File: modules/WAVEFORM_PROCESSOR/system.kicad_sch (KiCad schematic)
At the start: 8 parts, among them J1 Card_Connector, J2 Mono_Jack, J3 Mono_Jack, J4 Mono_Jack, J5 Mono_Jack

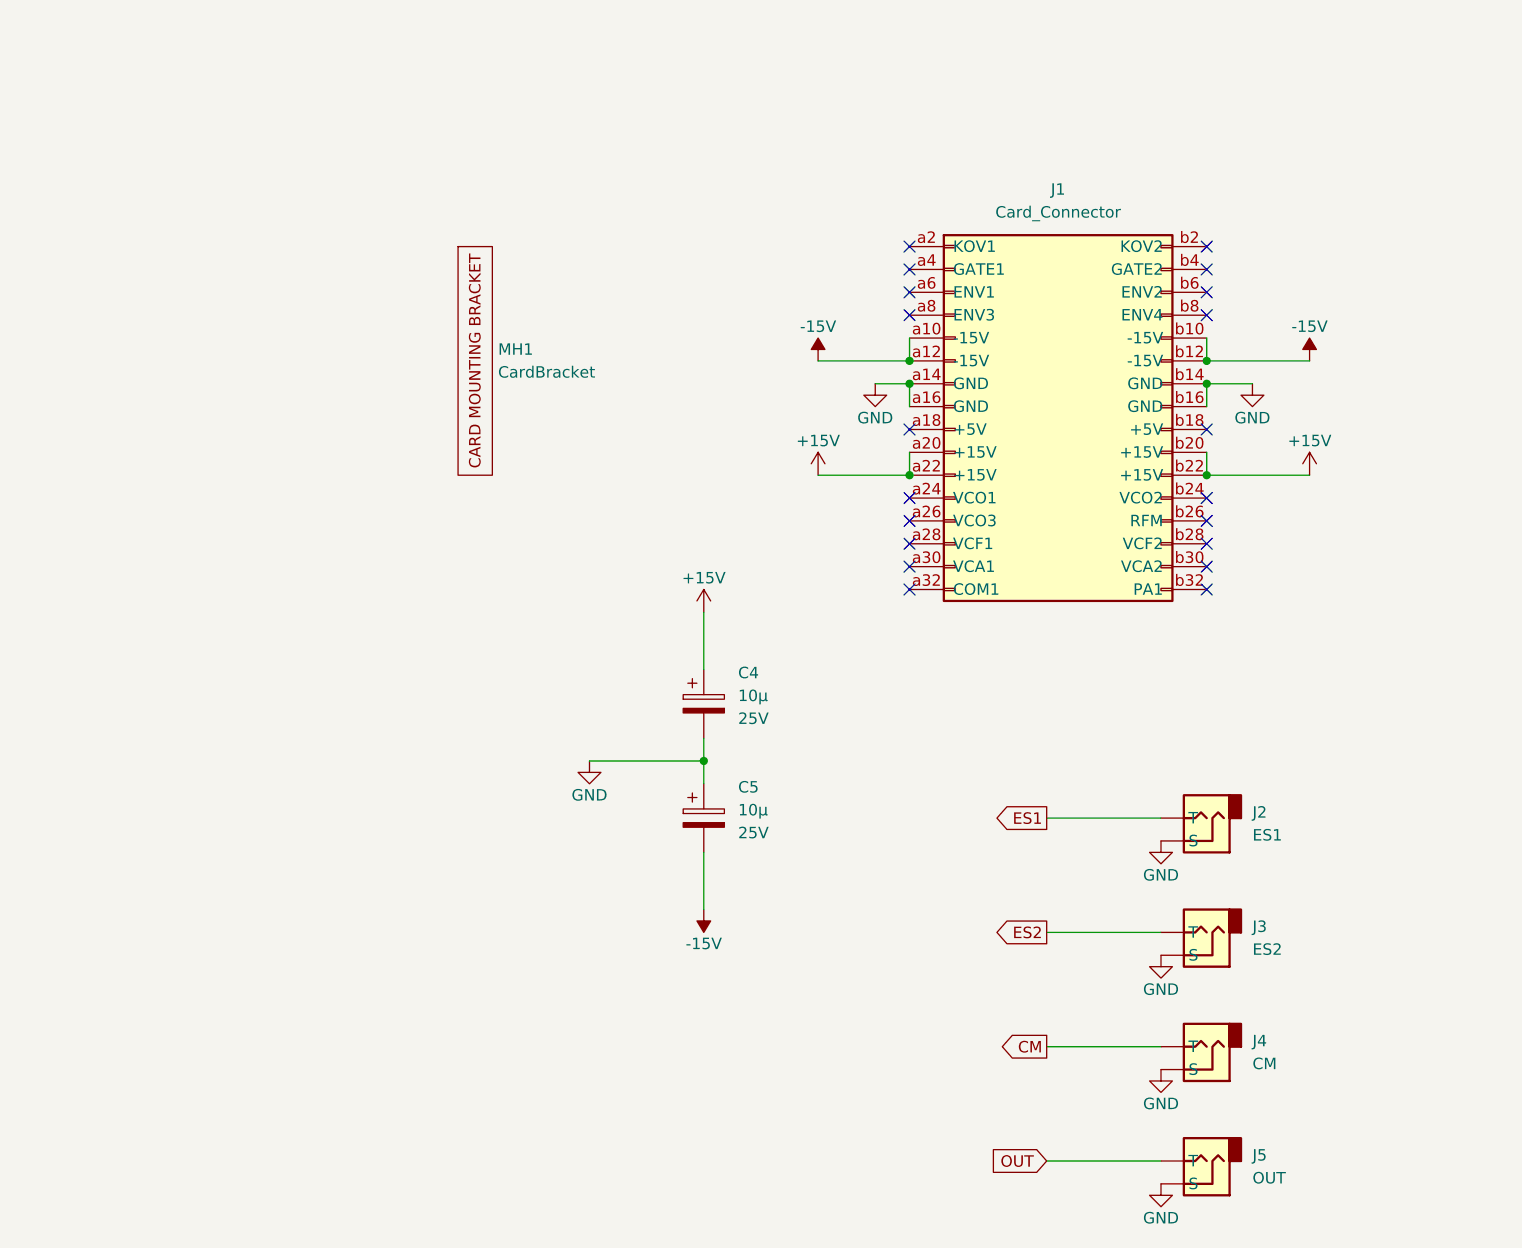
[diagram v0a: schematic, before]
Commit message: waveform processor updates
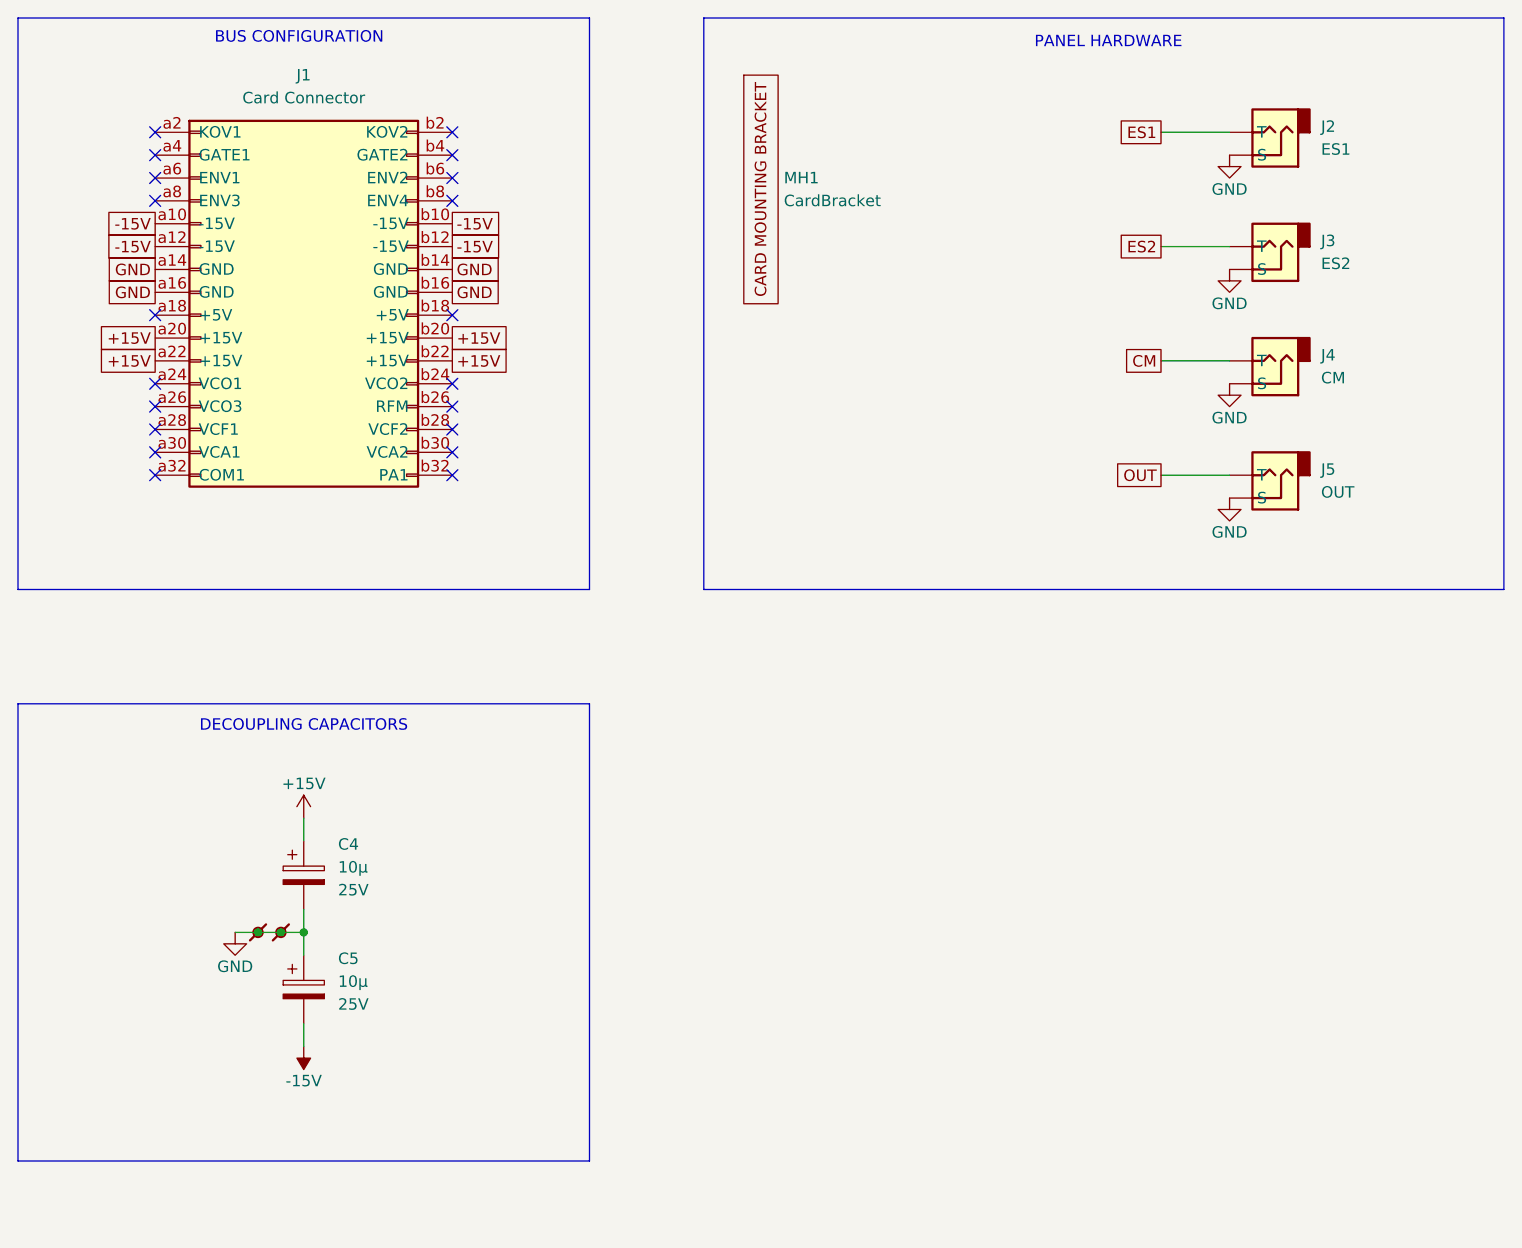
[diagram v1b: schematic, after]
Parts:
- added J7, J8: GND, FormantKO:Wire_1x01_D40mil_OD80mil, symbol FormantKO:WireConnector
- C4, C5: footprint FormantKO:CP_Axial_600 -> FormantKO:CP_Axial_P800mil
- J1: value Card_Connector -> Card Connector; footprint FormantKO:Card_Connector -> FormantKO:CardConnector; symbol FormantKO:Card_Connector -> FormantKO:CardConnector
- J2, J3, J4, J5: footprint FormantKO:Panel_Connector_1x02 -> FormantKO:PanelConnector_1x02; symbol FormantKO:Mono_Jack -> FormantKO:MonoJack
- MH1: footprint FormantKO:Card_Bracket -> FormantKO:CardBracket; symbol FormantKO:Card_Bracket -> FormantKO:CardBracket
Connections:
- net GND: now also J7.1, J8.1
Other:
- note added: "BUS CONFIGURATION"
- note added: "DECOUPLING CAPACITORS"
- note added: "PANEL HARDWARE"
- moved on the sheet: C4, C5, J1, J2, J3, J4, J5, MH1

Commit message: waveform process update
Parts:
- J7, J8: Spice_Model 0 -> (none); Spice_Primitive R -> (none)
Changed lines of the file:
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@@
 			)
 		)
-		(property "Spice_Primitive" "R"
+		(property "Sim.Device" "SPICE"
 			(at 55.245 125.73 0)
 			(hide yes)
@@
 			)
 		)
-		(property "Spice_Model" "0"
-			(at 52.705 128.905 0)
-			(hide yes)
-			(show_name no)
-			(do_not_autoplace no)
-			(effects
-				(font
-					(size 1.27 1.27)
-				)
-				(justify right top)
+		(property "Sim.Params" "type=\"R\" model=\"0\" lib=\"\""
+			(at 0 0 0)
+			(hide yes)
+			(show_name no)
+			(do_not_autoplace no)
+			(effects
+				(font
+					(size 1.27 1.27)
+				)
+			)
+		)
+		(property "Sim.Pins" "1=1"
+			(at 0 0 0)
+			(hide yes)
+			(show_name no)
+			(do_not_autoplace no)
+			(effects
+				(font
+					(size 1.27 1.27)
+				)
 			)
 		)
@@
 			)
 		)
-		(property "Spice_Primitive" "R"
+		(property "Sim.Device" "SPICE"
 			(at 52.705 125.73 0)
 			(hide yes)
@@
 			)
 		)
-		(property "Spice_Model" "0"
-			(at 50.165 128.905 0)
-			(hide yes)
-			(show_name no)
-			(do_not_autoplace no)
-			(effects
-				(font
-					(size 1.27 1.27)
-				)
-				(justify right top)
-			)
-		)
+		(property "Sim.Params" "type=\"R\" model=\"0\" lib=\"\""
+			(at 0 0 0)
+			(hide yes)
+			(show_name no)
+			(do_not_autoplace no)
+			(effects
+				(font
+					(size 1.27 1.27)
+				)
+			)
+		)
+		(property "Sim.Pins" "1=1"
+			(at 0 0 0)
+			(hide yes)
+			(show_name no)
+			(do_not_autoplace no)
+			(effects
+				(font
+					(size 1.27 1.27)
+				)
+			)
+		)

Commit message: mixer translation
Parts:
- C4, C5: footprint FormantKO:CP_Axial_P800mil -> FormantKO:CP_Axial_P600mil
- J7, J8: Spice_Model (none) -> 0; Spice_Primitive (none) -> R; now left out of the parts list
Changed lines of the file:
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@@
+			)
+		)
+		(property "Sim.Params" ""
+			(at 165.1 38.1 0)
+			(hide yes)
+			(show_name no)
+			(do_not_autoplace no)
+			(effects
+				(font
+					(size 1.27 1.27)
+				)
 			)
 		)
@@
 			)
 		)
+		(property "Sim.Params" ""
+			(at 165.1 76.2 0)
+			(hide yes)
+			(show_name no)
+			(do_not_autoplace no)
+			(effects
+				(font
+					(size 1.27 1.27)
+				)
+			)
+		)
 		(pin "1"
 		)
@@
 			)
 		)
+		(property "Sim.Params" ""
+			(at 165.1 63.5 0)
+			(hide yes)
+			(show_name no)
+			(do_not_autoplace no)
+			(effects
+				(font
+					(size 1.27 1.27)
+				)
+			)
+		)
 		(pin "1"
 		)
@@
 			)
 		)
+		(property "Sim.Params" ""
+			(at 107.95 44.45 0)
+			(hide yes)
+			(show_name no)
+			(do_not_autoplace no)
+			(effects
+				(font
+					(size 1.27 1.27)
+				)
+			)
+		)
 		(instances
 			(project "WAVEFORM_PROCESSOR"
@@
 			)
 		)
+		(property "Sim.Params" ""
+			(at 165.1 50.8 0)
+			(hide yes)
+			(show_name no)
+			(do_not_autoplace no)
+			(effects
+				(font
+					(size 1.27 1.27)
+				)
+			)
+		)
 		(pin "1"
 		)
@@
 		(body_style 1)
 		(exclude_from_sim no)
-		(in_bom yes)
+		(in_bom no)
 		(on_board yes)
 		(in_pos_files yes)
@@
 			)
 		)
-		(property "Sim.Device" "SPICE"
+		(property "Spice_Primitive" "R"
 			(at 55.245 125.73 0)
 			(hide yes)
@@
 			)
 		)
-		(property "Sim.Params" "type=\"R\" model=\"0\" lib=\"\""
-			(at 0 0 0)
-			(hide yes)
-			(show_name no)
-			(do_not_autoplace no)
-			(effects
-				(font
-					(size 1.27 1.27)
-				)
-			)
-		)
-		(property "Sim.Pins" "1=1"
-			(at 0 0 0)
+		(property "Spice_Model" "0"
+			(at 52.705 128.905 0)
+			(hide yes)
+			(show_name no)
+			(do_not_autoplace no)
+			(effects
+				(font
+					(size 1.27 1.27)
+				)
+				(justify right top)
+			)
+		)
+		(property "Sim.Params" ""
+			(at 54.61 127 0)
 			(hide yes)
 			(show_name no)
@@
 			)
 		)
+		(property "Sim.Params" ""
+			(at 57.15 57.15 0)
+			(hide yes)
+			(show_name no)
+			(do_not_autoplace no)
+			(effects
+				(font
+					(size 1.27 1.27)
+				)
+			)
+		)
 		(pin "b6"
 		)
@@
 		(body_style 1)
 		(exclude_from_sim no)
-		(in_bom yes)
+		(in_bom no)
 		(on_board yes)
 		(in_pos_files yes)
@@
 			)
 		)
-		(property "Sim.Device" "SPICE"
+		(property "Spice_Primitive" "R"
 			(at 52.705 125.73 0)
 			(hide yes)
@@
 			)
 		)
-		(property "Sim.Params" "type=\"R\" model=\"0\" lib=\"\""
-			(at 0 0 0)
-			(hide yes)
-			(show_name no)
-			(do_not_autoplace no)
-			(effects
-				(font
-					(size 1.27 1.27)
-				)
-			)
-		)
-		(property "Sim.Pins" "1=1"
-			(at 0 0 0)
+		(property "Spice_Model" "0"
+			(at 50.165 128.905 0)
+			(hide yes)
+			(show_name no)
+			(do_not_autoplace no)
+			(effects
+				(font
+					(size 1.27 1.27)
+				)
+				(justify right top)
+			)
+		)
+		(property "Sim.Params" ""
+			(at 52.07 127 0)
 			(hide yes)
 			(show_name no)
@@
 			)
 		)
-		(property "Footprint" "FormantKO:CP_Axial_P800mil"
+		(property "Footprint" "FormantKO:CP_Axial_P600mil"
 			(at 58.1152 124.46 0)
 			(hide yes)
@@
 				)
 				(justify left)
+			)
+		)
+		(property "Sim.Params" ""
+			(at 57.15 120.65 0)
+			(hide yes)
+			(show_name no)
+			(do_not_autoplace no)
+			(effects
+				(font
+					(size 1.27 1.27)
+				)
 			)
 		)
@@
 			)
 		)
-		(property "Footprint" "FormantKO:CP_Axial_P800mil"
+		(property "Footprint" "FormantKO:CP_Axial_P600mil"
 			(at 58.1152 137.16 0)
 			(hide yes)
@@
 			)
 		)
+		(property "Sim.Params" ""
+			(at 57.15 133.35 0)
+			(hide yes)
+			(show_name no)
+			(do_not_autoplace no)
+			(effects
+				(font
+					(size 1.27 1.27)
+				)
+			)
+		)
